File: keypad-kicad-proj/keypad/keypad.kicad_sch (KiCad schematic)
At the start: 14 parts, among them J1 Screw_Terminal_01x02, U1 ESP32-S3-WROOM-1, U2 TLV75901PDRVT

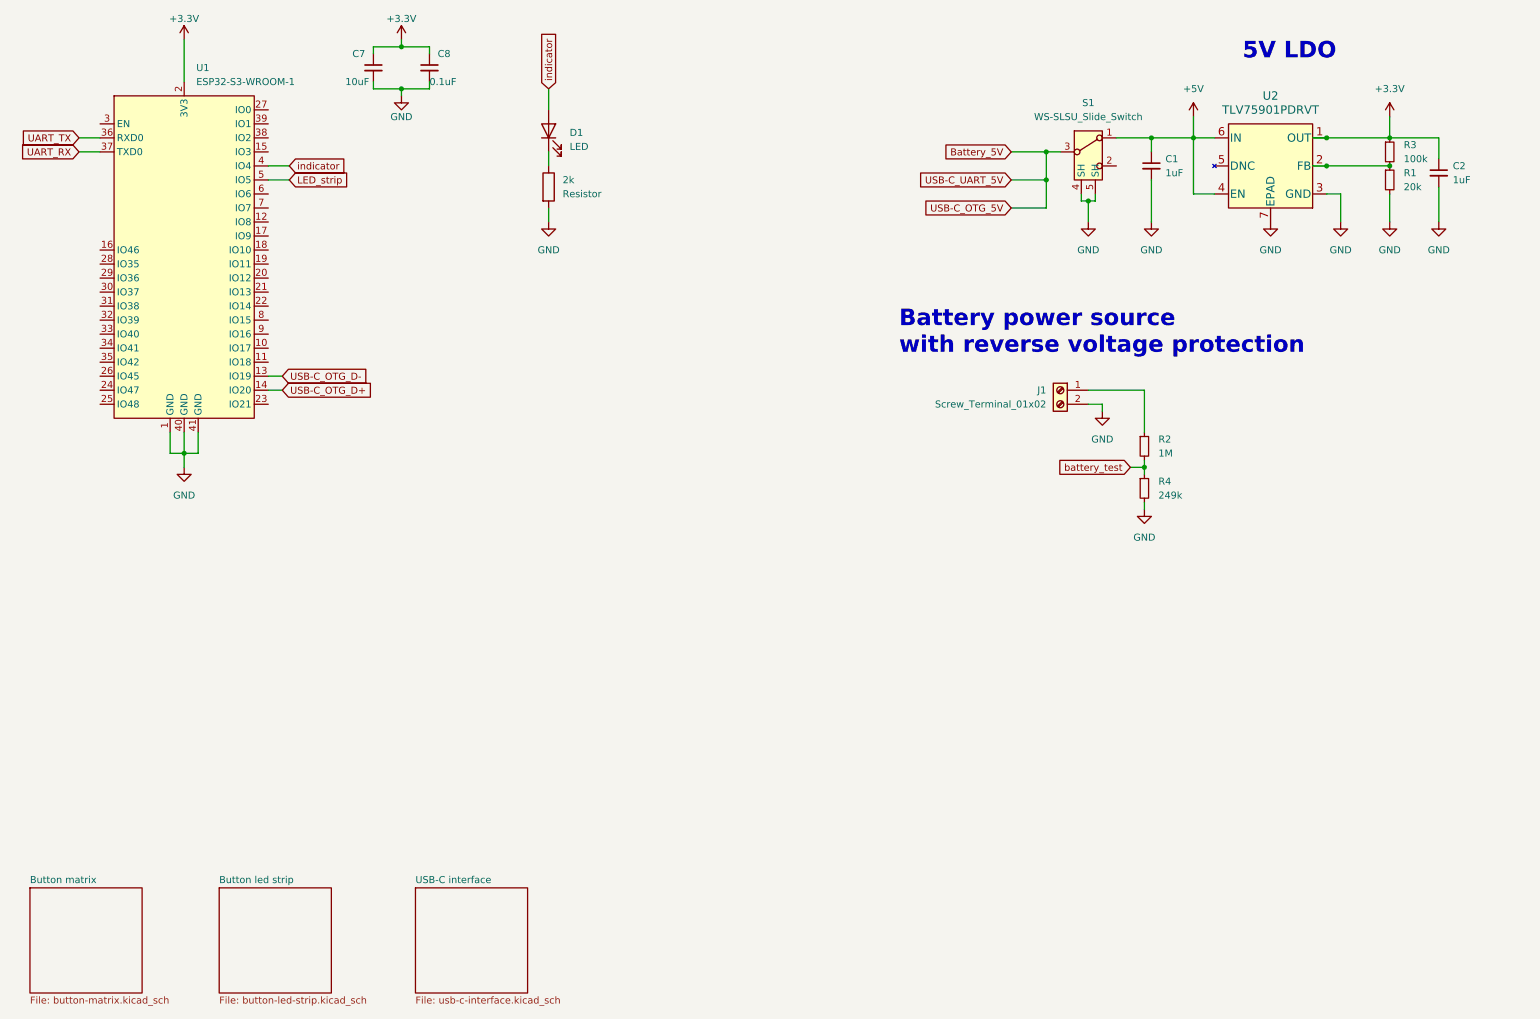
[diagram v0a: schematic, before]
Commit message: battery source
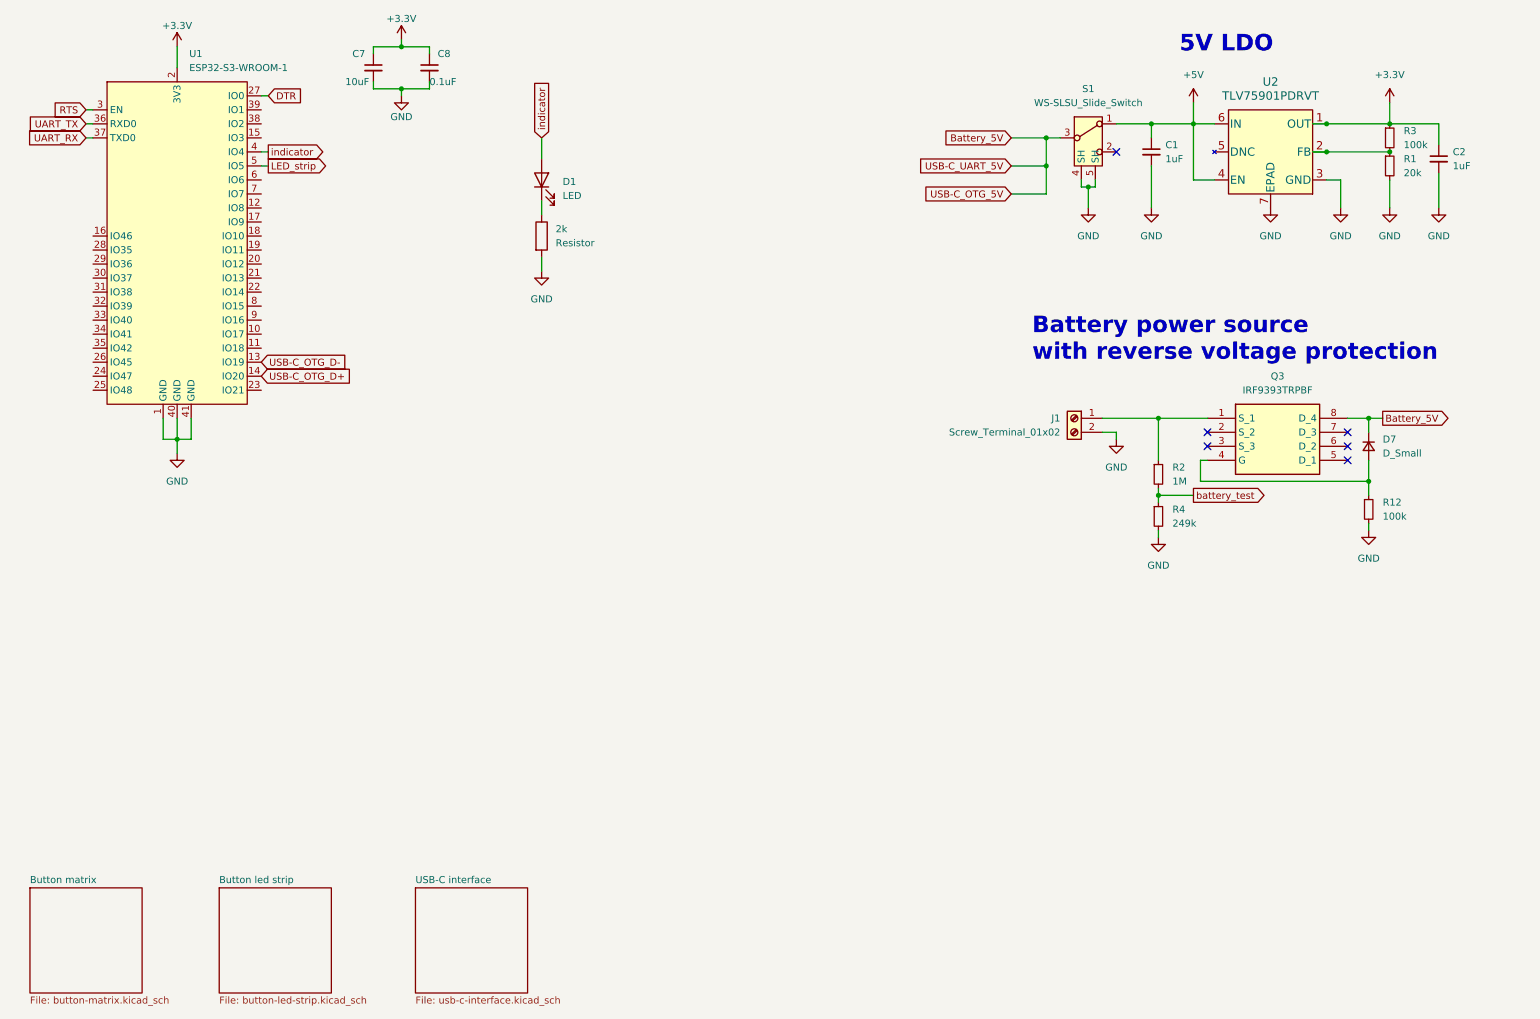
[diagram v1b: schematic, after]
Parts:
- added D7: D_Small, symbol Device:D_Small
- added Q3: IRF9393TRPBF, SOIC127P600X175-8N, symbol PUTRocketLab_semiconductors:IRF9393TRPBF
- added R12: 100k, symbol PutRocketLab_RCL:R_Small
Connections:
- net Battery_5V: now also D7.1 (K), Q3.8 (D_4)
- net GND: now also R12.2
- net DTR: now reaches U1.27 (IO0)
- net RTS: now reaches U1.3 (EN)
- net at J1.1 (Pin_1), R2.1: now also Q3.1 (S_1)
- new net: D7.2 (A), Q3.4 (G), R12.1
- no-connect marks 0 -> 6
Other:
- moved on the sheet: 2k, C1, C2, D1, J1, R1, R2, R3, R4, S1, U1, U2

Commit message: rest of the schematic
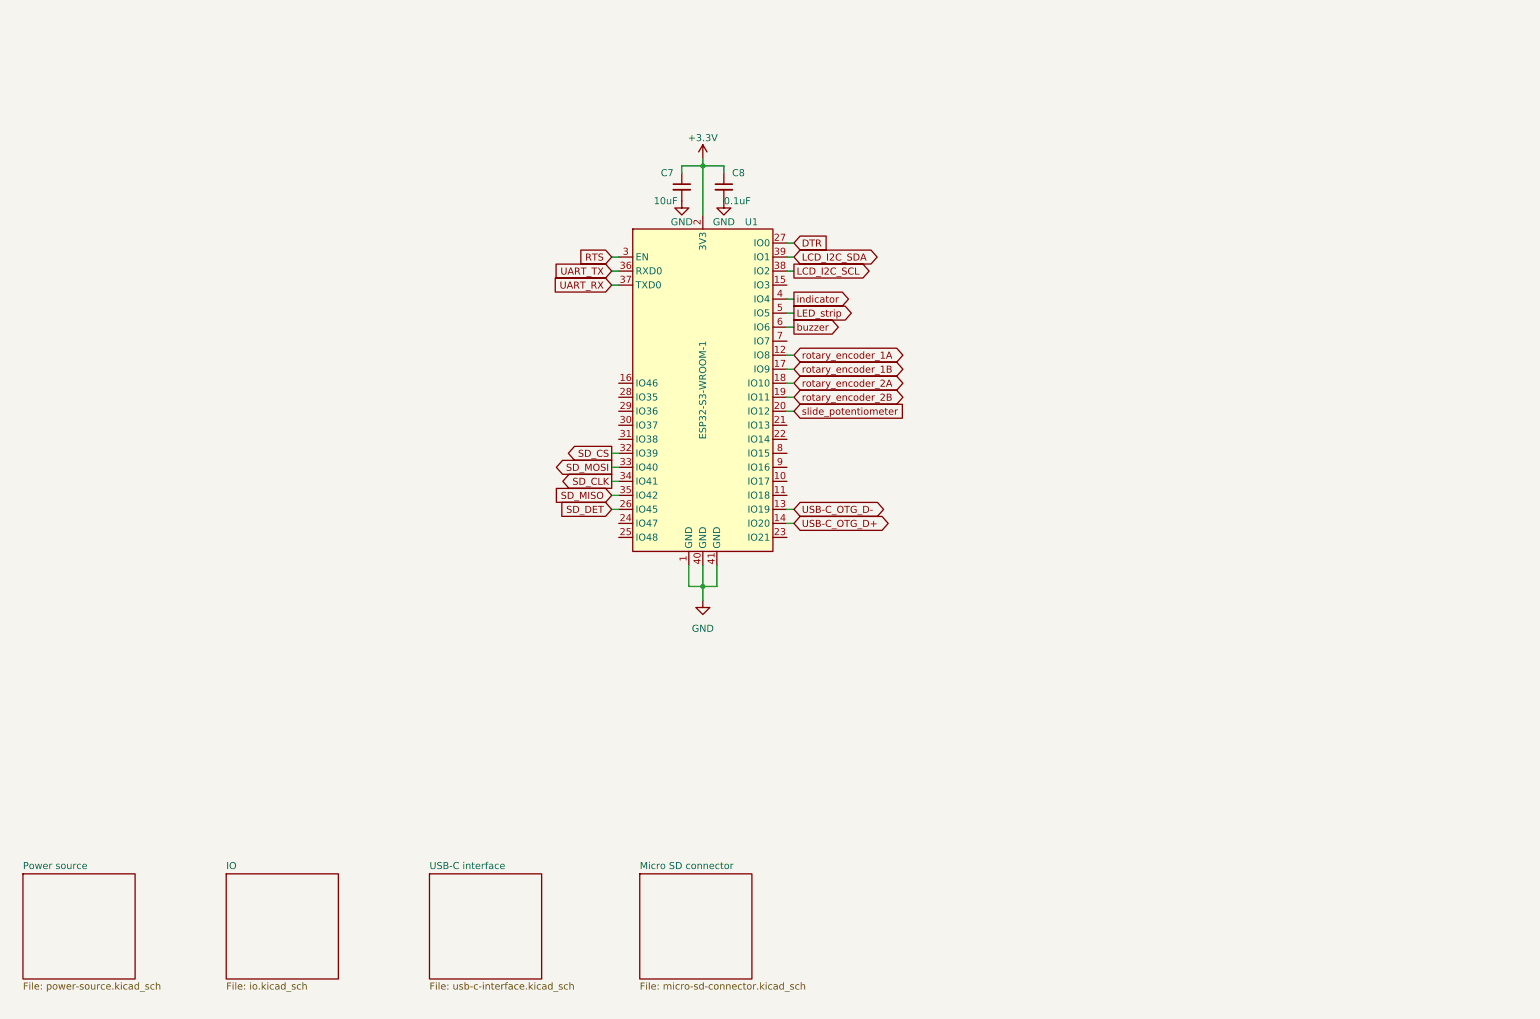
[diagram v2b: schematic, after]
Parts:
- removed 2k: Resistor, symbol PutRocketLab_RCL:Resistor
- removed C1, C2: 1uF, symbol PutRocketLab_RCL:C_Small
- removed D1: LED, symbol PUTRocketLab_semiconductors:LED
- removed D7: D_Small, symbol Device:D_Small
- removed J1: Screw_Terminal_01x02, symbol Connector:Screw_Terminal_01x02
- removed Q3: IRF9393TRPBF, SOIC127P600X175-8N, symbol PUTRocketLab_semiconductors:IRF9393TRPBF
- removed R1: 20k, symbol PutRocketLab_RCL:R_Small
- removed R12, R3: 100k, symbol PutRocketLab_RCL:R_Small
- removed R2: 1M, symbol PutRocketLab_RCL:R_Small
- removed R4: 249k, symbol PutRocketLab_RCL:R_Small
- removed S1: WS-SLSU_Slide_Switch, symbol PUT_RocketLab_connectors:WS-SLSU_Slide_Switch
- removed U2: TLV75901PDRVT, DRV6_1X1P6_TEX, symbol PUT_RocketLab_IC:TLV75901PDRVT
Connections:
- net rotary_encoder_1A: now reaches U1.12 (IO8)
- net rotary_encoder_1B: now reaches U1.17 (IO9)
- net rotary_encoder_2A: now reaches U1.18 (IO10)
- net rotary_encoder_2B: now reaches U1.19 (IO11)
- net slide_potentiometer: now reaches U1.20 (IO12)
- net SD_DET: now reaches U1.26 (IO45)
- net SD_CS: now reaches U1.32 (IO39)
- net SD_MOSI: now reaches U1.33 (IO40)
- net SD_CLK: now reaches U1.34 (IO41)
- net SD_MISO: now reaches U1.35 (IO42)
- net LCD_I2C_SCL: now reaches U1.38 (IO2)
- net LCD_I2C_SDA: now reaches U1.39 (IO1)
- net buzzer: now reaches U1.6 (IO6)
- no-connect marks 6 -> 0
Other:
- removed sheet Button led strip
- removed sheet Button matrix
- added sheet IO (io.kicad_sch)
- added sheet Micro SD connector (micro-sd-connector.kicad_sch)
- added sheet Power source (power-source.kicad_sch)
- note removed: "5V LDO"
- note removed: "Battery power source with reverse voltage protection"
- title: (none) -> Keypad board
- moved on the sheet: C7, U1
